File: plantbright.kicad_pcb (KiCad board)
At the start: 2 copper layers, 33 x 54 mm, 24 parts, among them J1 POWER OUT, J2 USB-C, Q1 AO3400A, Q2 AO3400A, Q3 AO3400A, Q5 AO3400A, SW1 USER 0, U1 XIAO-ESP32-C6

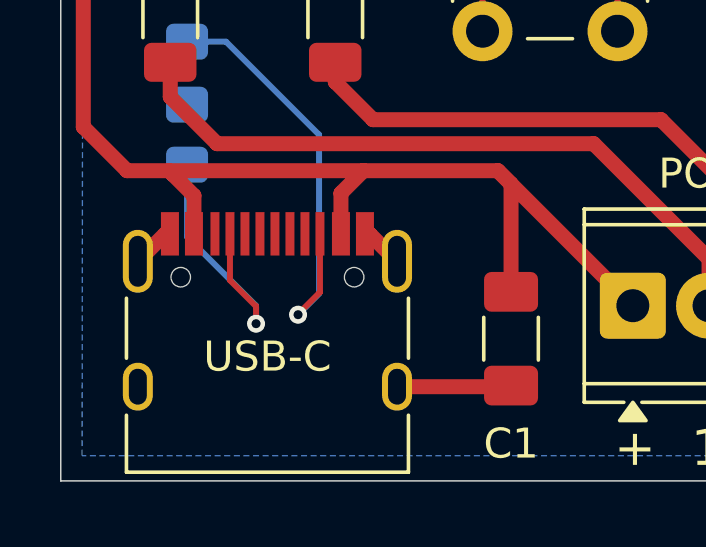
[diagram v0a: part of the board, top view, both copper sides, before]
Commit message: Update plantbright.kicad_pcb
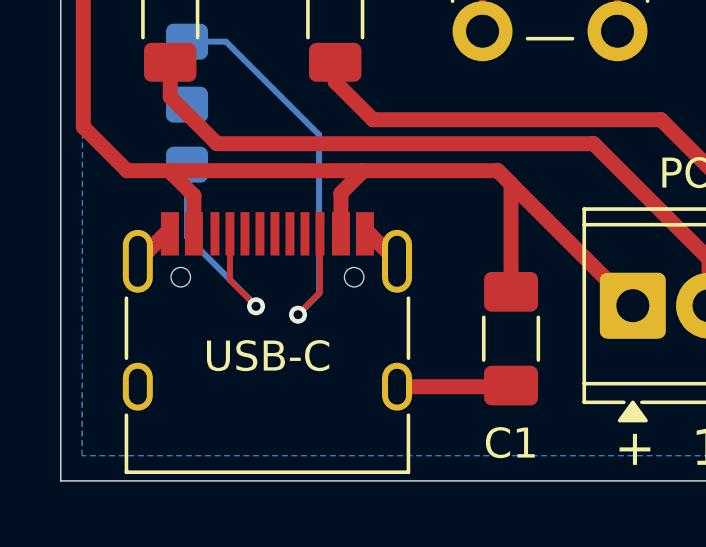
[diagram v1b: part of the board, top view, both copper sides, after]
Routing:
- net Net-(J2-CC1): track 9.61 -> 8.45 mm
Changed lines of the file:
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@@
-		(net 20)
-	)
-	(segment
-		(start 143.3 113.1)
-		(end 143.3 112.52)
-		(width 0.2)
-		(layer "F.Cu")
 		(net 20)
 	)
 	(via
-		(at 143.3 113.1)
+		(at 143.3 112.52)
 		(size 0.6)
 		(drill 0.3)
@@
 	)
 	(segment
-		(start 143.3 113.1)
-		(end 143.3 112.5)
+		(start 143.3 112.5)
+		(end 141 110.2)
 		(width 0.2)
 		(layer "B.Cu")
@@
 	)
 	(segment
-		(start 143.3 112.5)
-		(end 141 110.2)
+		(start 143.3 112.52)
+		(end 143.3 112.5)
 		(width 0.2)
 		(layer "B.Cu")
